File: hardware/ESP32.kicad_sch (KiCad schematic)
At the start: 17 parts, among them J1 USB_C_Receptacle_USB2.0_16P, SW1 SW_Omron_B3FS, SW2 SW_Omron_B3FS, U2 ESP32-C3-WROOM-02, U8 USBLC6-2SC6

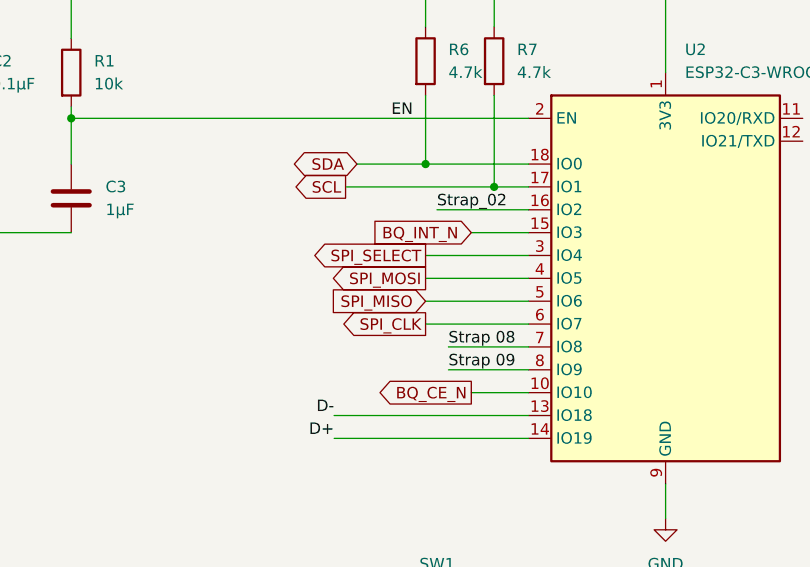
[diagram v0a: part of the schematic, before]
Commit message: Module Lora
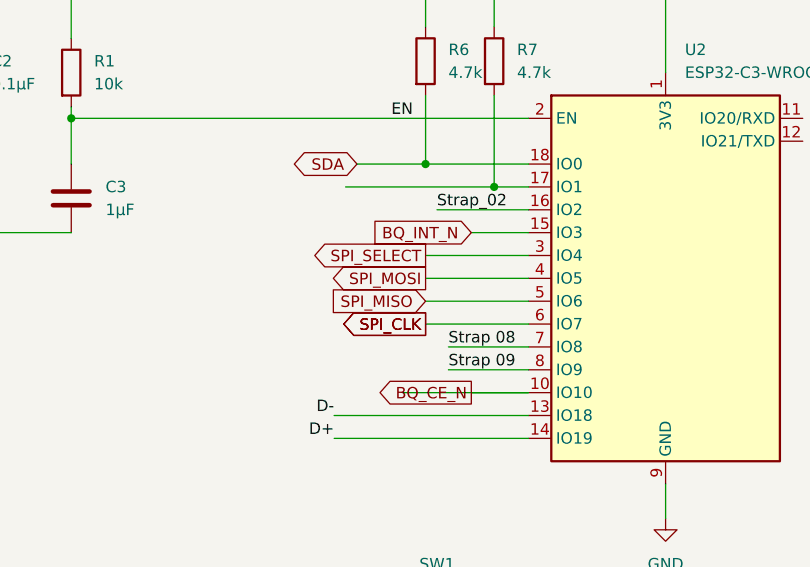
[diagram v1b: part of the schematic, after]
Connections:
- net SCL: no longer names the net of R7.2, U2.17 (IO1)
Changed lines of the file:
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@@
+	(wire
+		(pts
+			(xy 184.15 76.2) (xy 198.12 76.2)
+		)
+		(stroke
+			(width 0)
+			(type default)
+		)
+	)
 	(wire
 		(pts
@@
 		)
 		(property "Intersheetrefs" "${INTERSHEET_REFS}"
-			(at 176.0848 68.58 0)
+			(at 175.4197 76.2 0)
 			(effects
 				(font
@@
 		)
 	)
-	(global_label "SCL"
+	(global_label "SPI_CLK"
 		(shape output)
-		(at 177.8 53.34 180)
+		(at 186.69 68.58 180)
 		(fields_autoplaced yes)
 		(effects
@@
 		)
 		(property "Intersheetrefs" "${INTERSHEET_REFS}"
-			(at 171.3072 53.34 0)
+			(at 176.0848 68.58 0)
 			(effects
 				(font
